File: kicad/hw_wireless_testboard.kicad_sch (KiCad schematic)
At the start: 0 parts

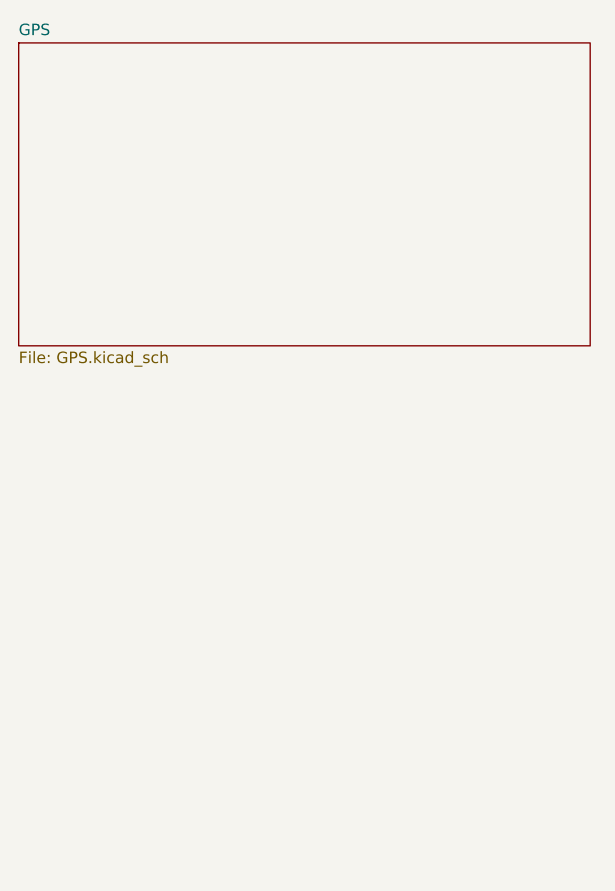
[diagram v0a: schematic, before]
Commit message: minor changes
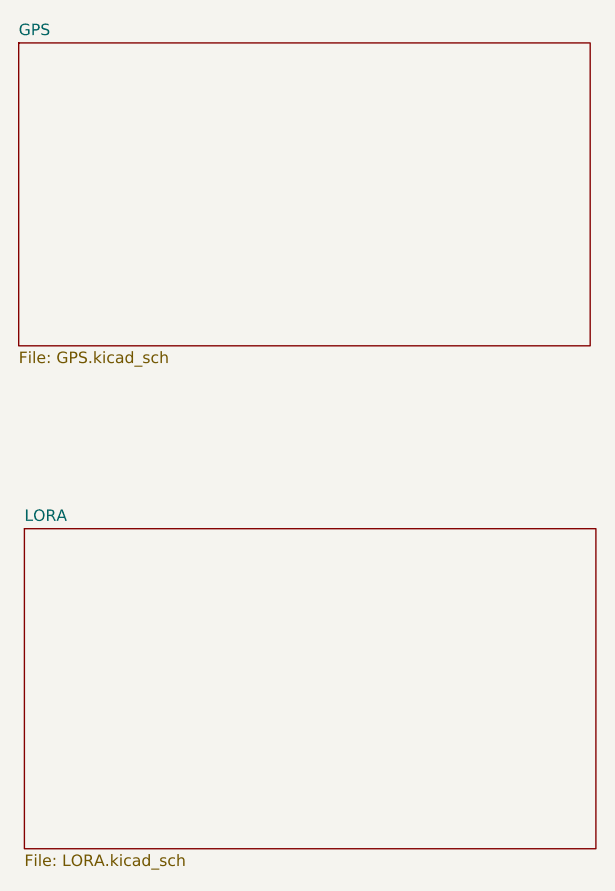
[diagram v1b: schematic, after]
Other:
- added sheet LORA (LORA.kicad_sch)
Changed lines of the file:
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@@
+		)
+	)
+	(sheet
+		(at 33.02 81.28)
+		(size 63.5 35.56)
+		(fields_autoplaced yes)
+		(stroke
+			(width 0.1524)
+			(type solid)
+		)
+		(fill
+			(color 0 0 0 0.0000)
+		)
+		(property "Sheetname" "LORA"
+			(at 33.02 80.5684 0)
+			(effects
+				(font
+					(size 1.27 1.27)
+				)
+				(justify left bottom)
+			)
+		)
+		(property "Sheetfile" "LORA.kicad_sch"
+			(at 33.02 117.4246 0)
+			(effects
+				(font
+					(size 1.27 1.27)
+				)
+				(justify left top)
+			)
+		)
+		(instances
+			(project "hw_wireless_testboard"
+				(path "/601a88ea-2da7-4ec4-b637-f587eb4ba821"
+					(page "3")
+				)
+			)
 		)
 	)
